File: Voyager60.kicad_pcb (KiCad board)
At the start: 2 copper layers, 285 x 95.1 mm, 265 parts, among them Q1 2N7002, SW1 5.2x5.2mm, U1 ATmega32U4-MU, U2 PRTR5V0U2X, Y1 16Mhz

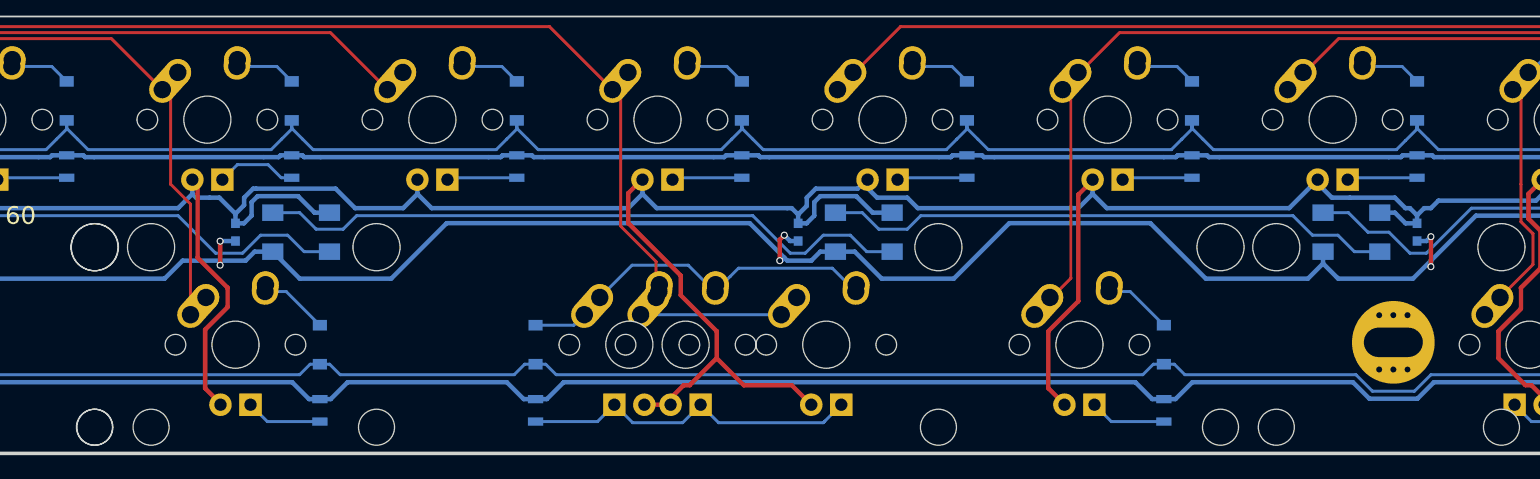
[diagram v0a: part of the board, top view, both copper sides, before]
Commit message: start changes
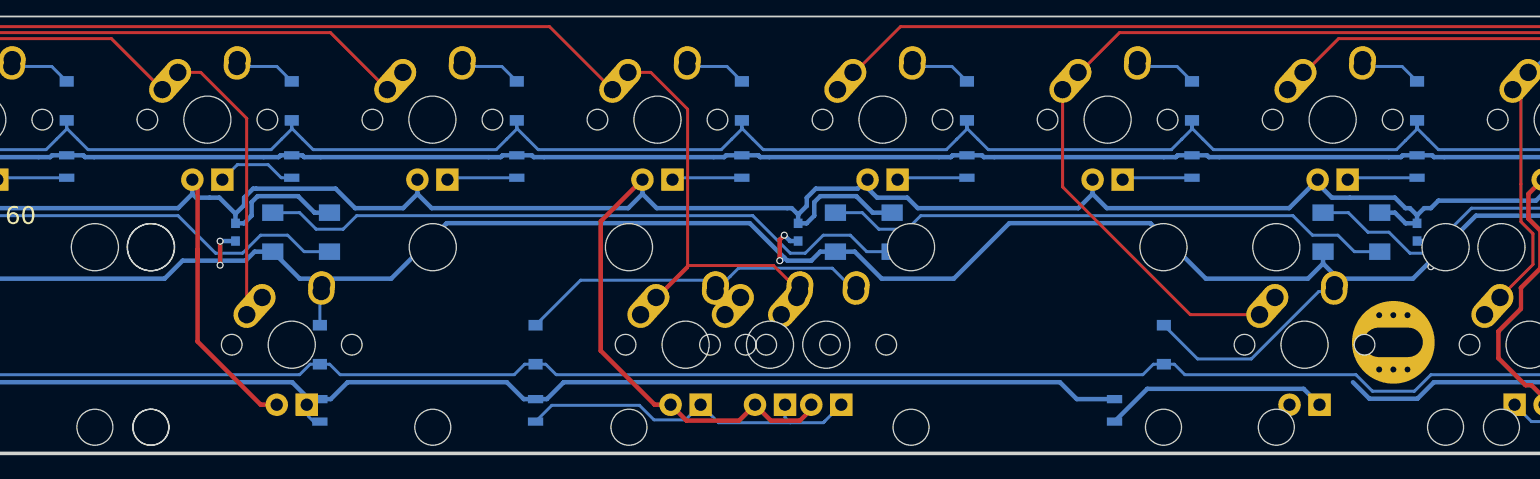
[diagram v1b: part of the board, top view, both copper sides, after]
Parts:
- K_SPACE5: value MX-1.25U -> 2U; footprint MX_Alps_Hybrid:MX-1.25U-FLIPPED -> MX_Alps_Hybrid:MX-2U-ReversedStabilizers
- moved K_SPACE4 19.1 mm to (205.6, 108.0)
- moved K_SPACE5 11.9 mm to (160.3, 108.0)
- moved K_SPACE3 4.76 mm to (119.9, 108.0)
- moved R62 4.18 mm to (189.5, 113.5)
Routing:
- net LEDGND: track 1409.4 -> 1388.6 mm
- net +5V: track 1795.4 -> 1778.4 mm
- net COL6: track 369.3 -> 382.5 mm
- net Net-(K_SPACE4-Pad4): track 6.46 -> 19.1 mm
- net Net-(D62-Pad2): track 5.82 -> 18.0 mm
- net COL8: track 365.8 -> 375.5 mm
- net Net-(K_SPACE3-Pad4): track 6.46 -> 1.18 mm
- net COL4: track 243.6 -> 248.6 mm
- net Net-(D58-Pad2): track 5.82 -> 2.90 mm
- net Net-(K_SPACE1-Pad4): track 29.0 -> 30.5 mm
- net Net-(D61-Pad2): track 29.9 -> 30.6 mm
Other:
- net class Default removed
- net class Power removed
